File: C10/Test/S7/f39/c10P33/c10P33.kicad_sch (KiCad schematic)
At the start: 5 parts

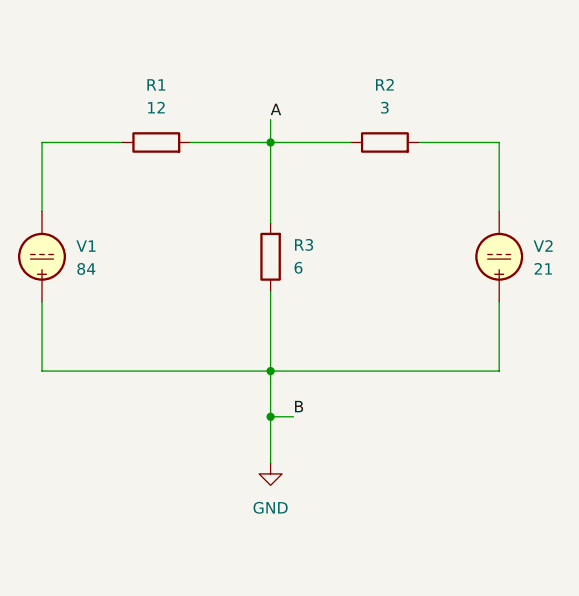
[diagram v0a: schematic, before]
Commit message: additiona upload Chapter 10
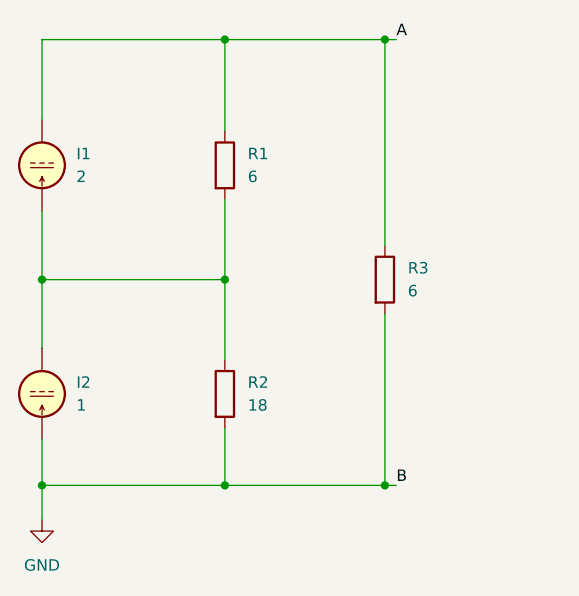
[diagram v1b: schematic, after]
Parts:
- removed V1: 84, symbol Simulation_SPICE:VDC
- removed V2: 21, symbol Simulation_SPICE:VDC
- added I1: 2, symbol Simulation_SPICE:IDC
- added I2: 1, symbol Simulation_SPICE:IDC
- R1: value 12 -> 6
- R2: value 3 -> 18
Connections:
- net A: now also R1.1, R3.1, I1.2; no longer R1.2, R2.1, R3.2
- net GND: now also R2.2, R3.2, I2.1; no longer R3.1
- new net: I1.1, I2.2, R1.2, R2.1
